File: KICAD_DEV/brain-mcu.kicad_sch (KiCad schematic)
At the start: 21 parts, among them SW1 SW_Push, SW2 SW_Push, U1 STM32H743VITx, Y1 8 MHz, Y2 32.768 KHz

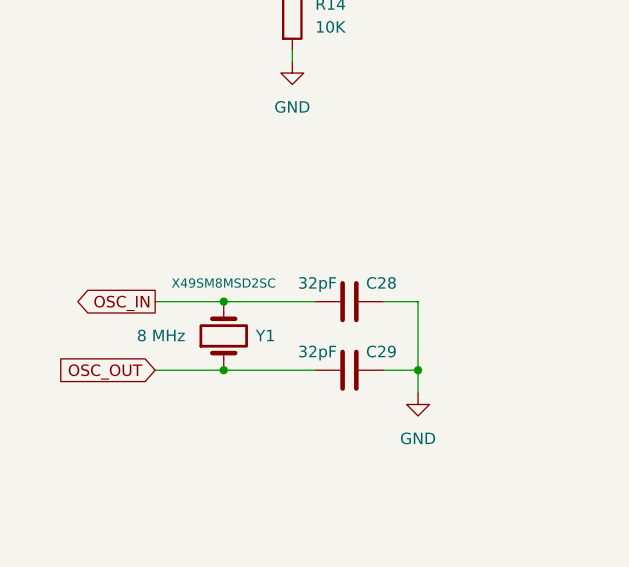
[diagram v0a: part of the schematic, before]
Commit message: assigning more footprints!g
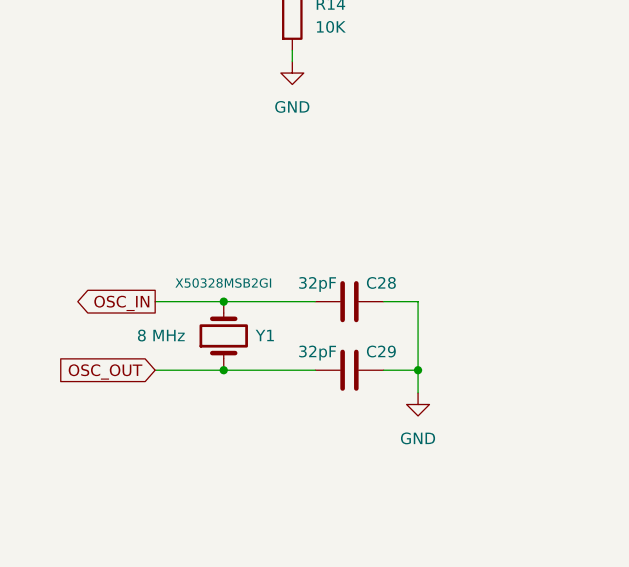
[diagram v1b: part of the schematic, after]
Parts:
- Y1: footprint (none) -> Crystal:Crystal_SMD_TXC_7A-2Pin_5x3.2mm; Part X49SM8MSD2SC -> X50328MSB2GI
- Y2: footprint (none) -> Crystal:Crystal_SMD_3215-2Pin_3.2x1.5mm
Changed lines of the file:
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@@
 			)
 		)
-		(property "Footprint" ""
+		(property "Footprint" "Crystal:Crystal_SMD_3215-2Pin_3.2x1.5mm"
 			(at 68.58 213.36 0)
 			(effects
@@
 			)
 		)
-		(property "Footprint" ""
+		(property "Footprint" "Crystal:Crystal_SMD_TXC_7A-2Pin_5x3.2mm"
 			(at 68.58 179.07 0)
 			(effects
@@
 			)
 		)
-		(property "Part" "X49SM8MSD2SC"
+		(property "Part" "X50328MSB2GI"
 			(at 68.58 173.228 90)
 			(effects
